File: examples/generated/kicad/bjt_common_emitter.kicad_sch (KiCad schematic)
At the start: 11 parts, among them Q1 2N3904

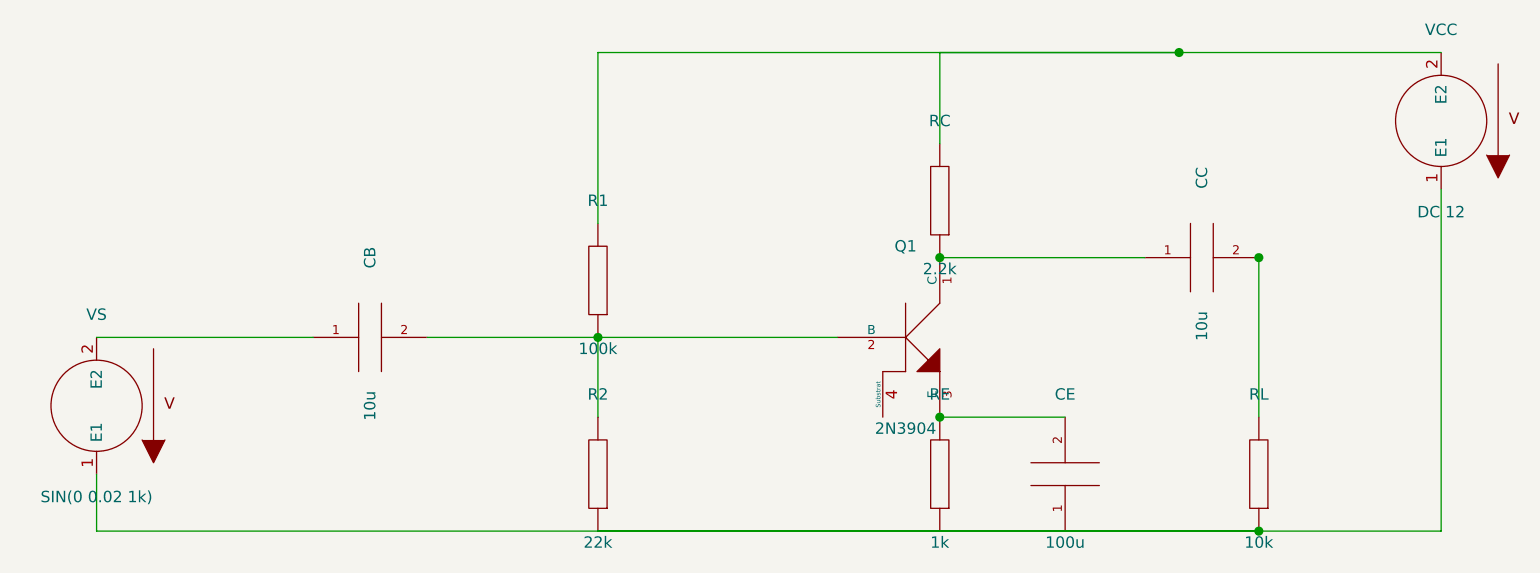
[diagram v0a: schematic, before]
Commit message: Refactor further.
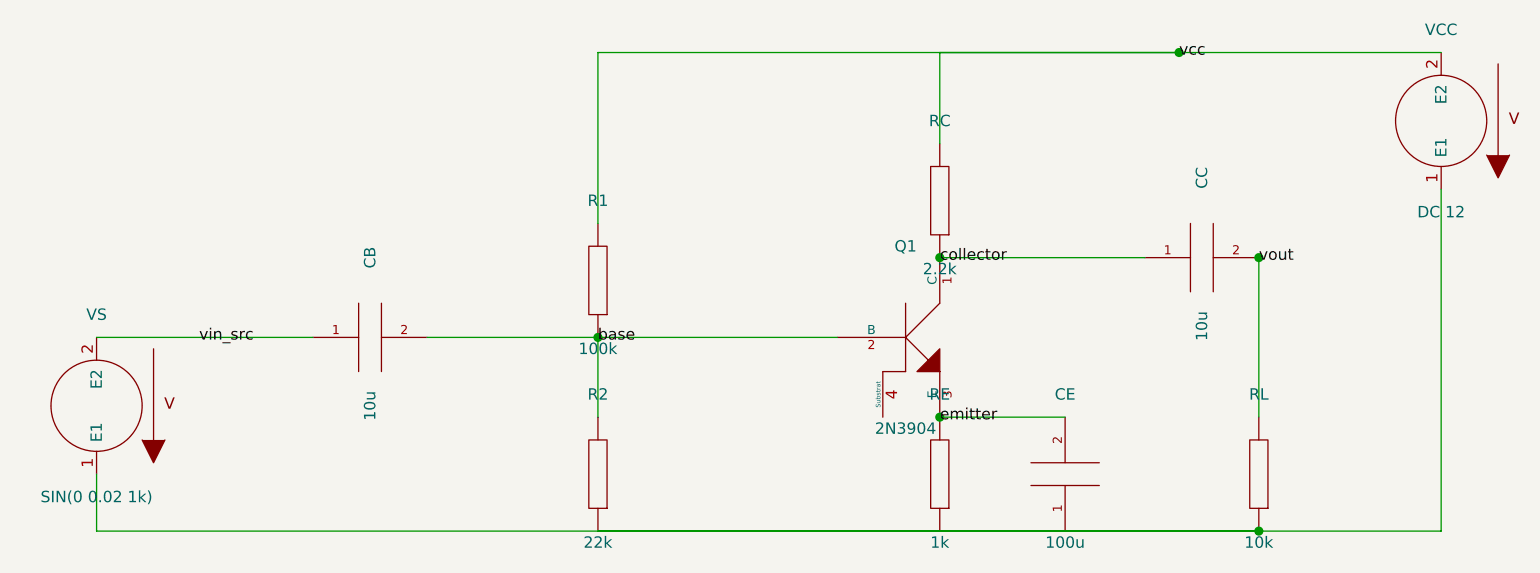
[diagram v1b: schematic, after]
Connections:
- net vout: now reaches CC.2, RL.2
- net vin_src: now reaches CB.1, VS.2 (E2)
- net emitter: now reaches CE.2, Q1.3 (E), RE.2
- net collector: now reaches CC.1, Q1.1 (C), RC.1
- net base: now reaches CB.2, Q1.2 (B), R1.1, R2.2
- net vcc: now reaches R1.2, RC.2, VCC.2 (E2)
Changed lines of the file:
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@@
     )
+  )
+  (label "vcc" (at 190.50 68.58 0)
+    (effects (font (size 1.27 1.27)))
+  )
+  (label "base" (at 125.73 100.33 0)
+    (effects (font (size 1.27 1.27)))
+  )
+  (label "vin_src" (at 81.28 100.33 0)
+    (effects (font (size 1.27 1.27)))
+  )
+  (label "collector" (at 163.83 91.44 0)
+    (effects (font (size 1.27 1.27)))
+  )
+  (label "emitter" (at 163.83 109.22 0)
+    (effects (font (size 1.27 1.27)))
+  )
+  (label "vout" (at 199.39 91.44 0)
+    (effects (font (size 1.27 1.27)))
   )
   (wire (pts (xy 219.71 68.58) (xy 190.50 68.58))

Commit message: Attempt substrate grounding.
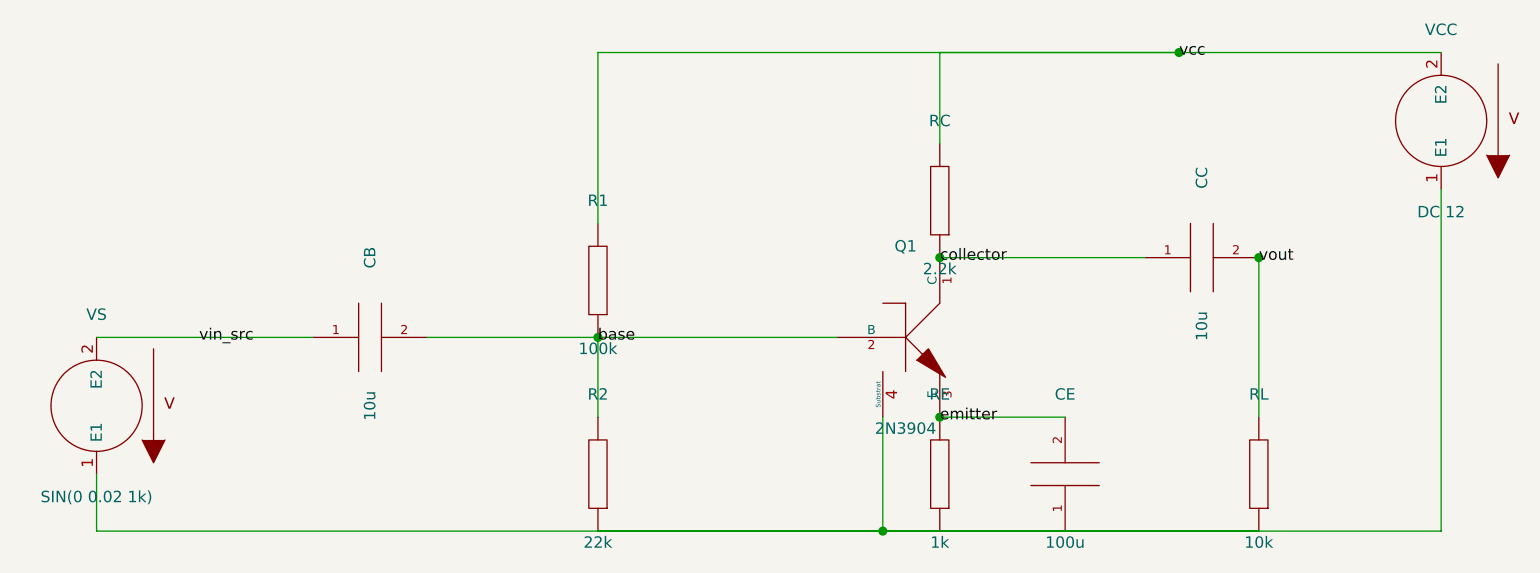
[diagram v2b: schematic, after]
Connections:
- net at CE.1, R2.1, RE.1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: now also Q1.4 (Substrat)
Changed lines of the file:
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@@
   (title_block
     (title "bjt_common_emitter")
-    (date "2026-03-07")
+    (date "2026-03-13")
     (comment 1 "Generated by mixedsig2cad")
   )
@@
     (stroke (width 0) (type solid) (color 0 0 0 0))
   )
-  (wire (pts (xy 69.85 121.92) (xy 199.39 121.92))
-    (stroke (width 0) (type solid) (color 0 0 0 0))
-  )
-  (wire (pts (xy 125.73 121.92) (xy 199.39 121.92))
-    (stroke (width 0) (type solid) (color 0 0 0 0))
-  )
-  (wire (pts (xy 163.83 121.92) (xy 199.39 121.92))
-    (stroke (width 0) (type solid) (color 0 0 0 0))
-  )
-  (wire (pts (xy 177.80 121.92) (xy 199.39 121.92))
+  (wire (pts (xy 69.85 121.92) (xy 157.48 121.92))
+    (stroke (width 0) (type solid) (color 0 0 0 0))
+  )
+  (wire (pts (xy 125.73 121.92) (xy 157.48 121.92))
+    (stroke (width 0) (type solid) (color 0 0 0 0))
+  )
+  (wire (pts (xy 163.83 121.92) (xy 157.48 121.92))
+    (stroke (width 0) (type solid) (color 0 0 0 0))
+  )
+  (wire (pts (xy 177.80 121.92) (xy 157.48 121.92))
+    (stroke (width 0) (type solid) (color 0 0 0 0))
+  )
+  (wire (pts (xy 199.39 121.92) (xy 157.48 121.92))
     (stroke (width 0) (type solid) (color 0 0 0 0))
   )
@@
     (stroke (width 0) (type solid) (color 0 0 0 0))
   )
-  (wire (pts (xy 219.71 121.92) (xy 199.39 121.92))
+  (wire (pts (xy 219.71 121.92) (xy 157.48 121.92))
+    (stroke (width 0) (type solid) (color 0 0 0 0))
+  )
+  (wire (pts (xy 157.48 109.22) (xy 157.48 121.92))
     (stroke (width 0) (type solid) (color 0 0 0 0))
   )
@@
   )
   (junction (at 190.50 68.58) (diameter 1.016) (color 0 0 0 0))
-  (junction (at 199.39 121.92) (diameter 1.016) (color 0 0 0 0))
+  (junction (at 157.48 121.92) (diameter 1.016) (color 0 0 0 0))
   (junction (at 125.73 100.33) (diameter 1.016) (color 0 0 0 0))
   (junction (at 163.83 91.44) (diameter 1.016) (color 0 0 0 0))

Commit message: Attempt to fix routing issues.
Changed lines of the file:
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@@
     (stroke (width 0) (type solid) (color 0 0 0 0))
   )
-  (wire (pts (xy 199.39 109.22) (xy 199.39 91.44))
+  (wire (pts (xy 199.39 91.44) (xy 199.39 109.22))
     (stroke (width 0) (type solid) (color 0 0 0 0))
   )
